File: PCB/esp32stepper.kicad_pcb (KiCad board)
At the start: 4 copper layers, 100 x 80 mm, 117 parts, among them J1 Conn_01x02_Pin, J4 spare, J5 UART0 DEBUG, U1 ESP32-S3-WROOM-2, U2 LDL1117_SOT223, U3 LT8610, U4 74HC595D, U5 USBLC6-2SC6, U6 TCA9548APWR

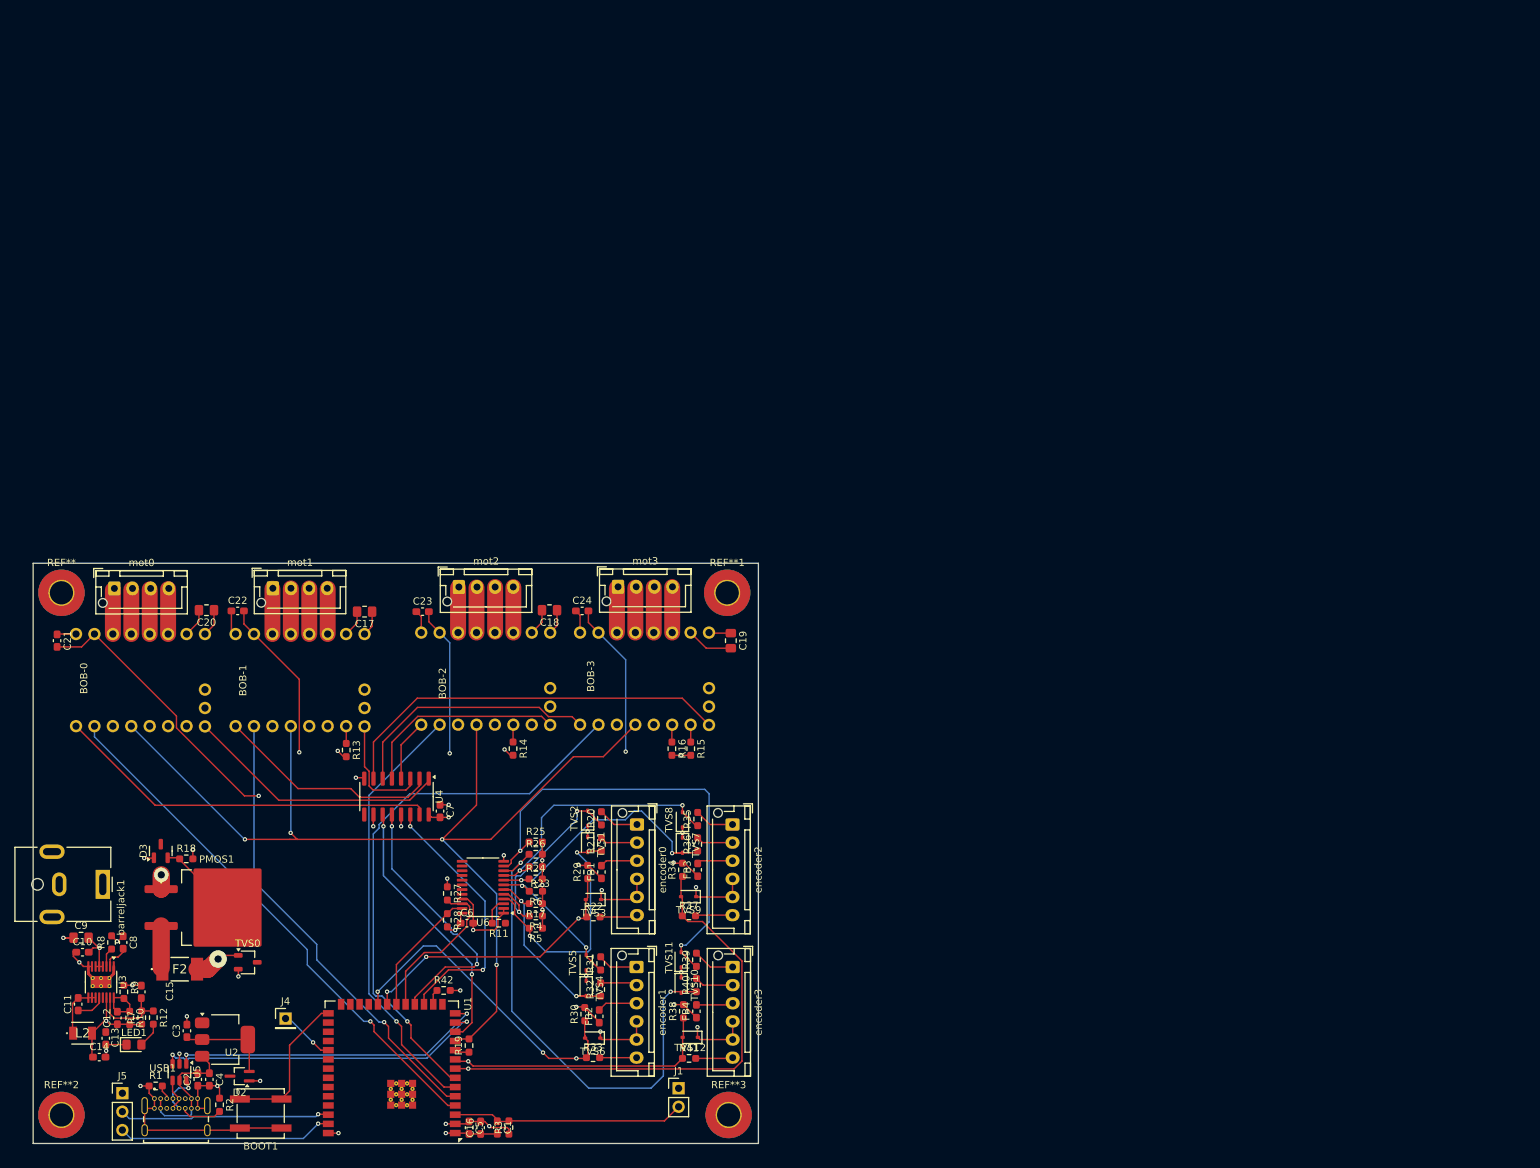
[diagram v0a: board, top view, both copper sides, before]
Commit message: pcb version ready for final check
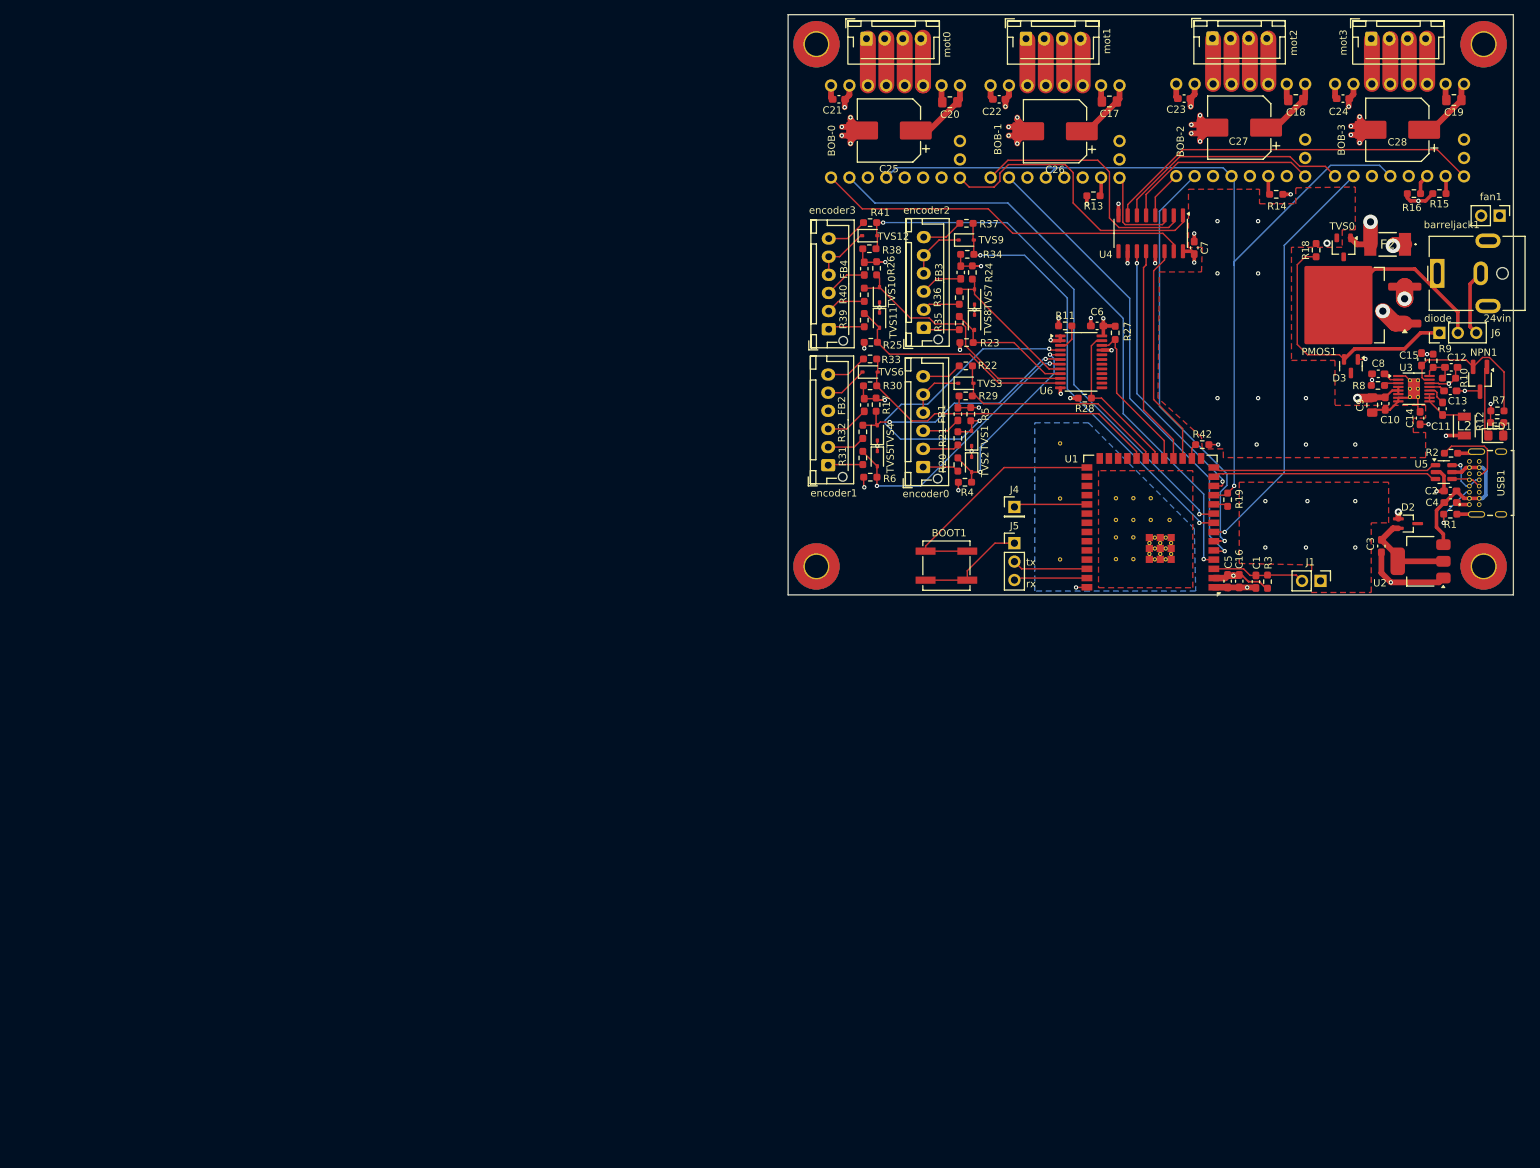
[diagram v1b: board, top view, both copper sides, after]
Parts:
- added ?: , , F.Cu at (200.4, 164.2)
- added ?: , , F.Cu at (198.0, 169.6)
- added ?: , , F.Cu at (190.3, 161.2)
- added ?: , , F.Cu at (198.0, 164.2)
- added ?: , , F.Cu at (205.4, 164.2)
- added ?: , , F.Cu at (200.4, 161.2)
- added ?: , , F.Cu at (190.3, 169.6)
- added ?: , , F.Cu at (198.0, 166.6)
- added ?: , , F.Cu at (190.3, 153.6)
- added ?: , , F.Cu at (198.0, 161.2)
- added ?: , , F.Cu at (200.4, 166.6)
- added ?: , , F.Cu at (200.4, 169.6)
- added ?: , , F.Cu at (202.8, 161.2)
- added ?: , , F.Cu at (202.8, 164.2)
- added C25: 100uF/50V, Capacitor_SMD:CP_Elec_8x10.5, F.Cu at (166.7, 110.5)
- added C26: 100uF/50V, Capacitor_SMD:CP_Elec_8x10.5, F.Cu at (189.6, 110.6)
- added C27: 100uF/50V, Capacitor_SMD:CP_Elec_8x10.5, F.Cu at (215.0, 110.1)
- added C28: 100uF/50V, Capacitor_SMD:CP_Elec_8x10.5, F.Cu at (236.8, 110.4)
- added J6: PWR_SWITCH, Connector_PinHeader_2.54mm:PinHeader_1x03_P2.54mm_Vertical, F.Cu at (242.6, 138.4)
- added NPN1: BC817-40, Package_TO_SOT_SMD:TSOT-23_HandSoldering, F.Cu at (248.2, 144.8)
- added REF**: IEAP_LOGO, VNfootprints:IEAP_LOGO, F.Cu at (212.6, 138.6)
- added fan1: Conn_01x02_Pin, Connector_PinHeader_2.54mm:PinHeader_1x02_P2.54mm_Vertical, F.Cu at (250.9, 122.2)
- moved L2 208.1 mm to (246.0, 151.2), turned to -90 degrees
- moved C13 205.8 mm to (244.1, 146.4), turned to 0 degrees
- moved LED1 205.7 mm to (250.4, 152.6)
- moved C11 205.3 mm to (243.0, 148.9), turned to -90 degrees
- moved R7 204.8 mm to (250.6, 149.2), turned to 0 degrees
- moved C12 204.6 mm to (244.2, 143.1), turned to 180 degrees
- moved USB1 203.3 mm to (251.1, 159.1), turned to 90 degrees
- moved R12 202.6 mm to (250.5, 150.8), turned to 0 degrees
- moved barreljack1 202.4 mm to (242.3, 130.2), turned to 90 degrees
- moved C14 202.3 mm to (239.9, 150.1), turned to 90 degrees
- moved R10 202.2 mm to (243.9, 144.6), turned to 0 degrees
- moved R9 200.4 mm to (241.7, 142.2)
- moved U3 198.7 mm to (239.1, 146.1), turned to 0 degrees
- moved C15 196.9 mm to (240.1, 142.0)
- moved R1 195.1 mm to (244.1, 163.4), turned to 180 degrees
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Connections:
- C15 pad 2: Net-(U3-PG) -> Net-(NPN1-B)
- D3 pad 2: Net-(D3-A) -> PWRSWITCH_diode
- F2 pad 1: Net-(PMOS1-S) -> Net-(PMOS1-D)
- LED1 pad 1: GND -> Net-(LED1-K)
- PMOS1 pad 1: 24Vin -> Net-(PMOS1-D)
- PMOS1 pad 2: Net-(D3-A) -> PWRSWITCH_gate
- PMOS1 pad 3: Net-(PMOS1-S) -> 24Vin
- R12 pad 1: Net-(U3-PG) -> +3V3
- R18 pad 1: Net-(D3-A) -> PWRSWITCH_diode
- R7 pad 2: Net-(U3-PG) -> Net-(NPN1-B)
- U3 pad 15: Net-(U3-PG) -> Net-(NPN1-B)
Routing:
- net +3V3: track 173.0 -> 82.1 mm, vias 22 -> 26
- net endswitch3: track 37.8 -> 74.6 mm, vias 1 -> 2
- net PWRSWITCH_diode: track 0.00 -> 36.0 mm
- net encoder3_SC: track 64.9 -> 32.6 mm, vias 2 -> 0
- net encoder3_SD: track 67.0 -> 35.7 mm, vias 2 -> 0
- net PWRSWITCH_gate: track 0.00 -> 26.8 mm
- net UART: track 150.5 -> 124.9 mm, vias 4 -> 1
- net 24V: track 27.7 -> 50.2 mm
- net Net-(NPN1-B): track 0.00 -> 21.7 mm
- net rx_ext: track 29.7 -> 10.1 mm, vias 1 -> 0
- net reset: track 32.2 -> 12.9 mm
- net step3: track 76.8 -> 57.9 mm
- net tx_ext: track 29.1 -> 10.4 mm, vias 1 -> 0
- net encoder2_SC: track 36.5 -> 18.5 mm, vias 2 -> 0
- net encoder1_SC: track 20.3 -> 37.9 mm
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- added copper zone on B.Cu, net GND
- added copper zone on F.Cu, net GND
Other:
- board text added: "24vin"
- board text added: "diode"
- board text added: "rx"
- board text added: "tx"
